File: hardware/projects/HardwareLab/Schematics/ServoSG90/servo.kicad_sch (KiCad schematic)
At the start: 2 parts

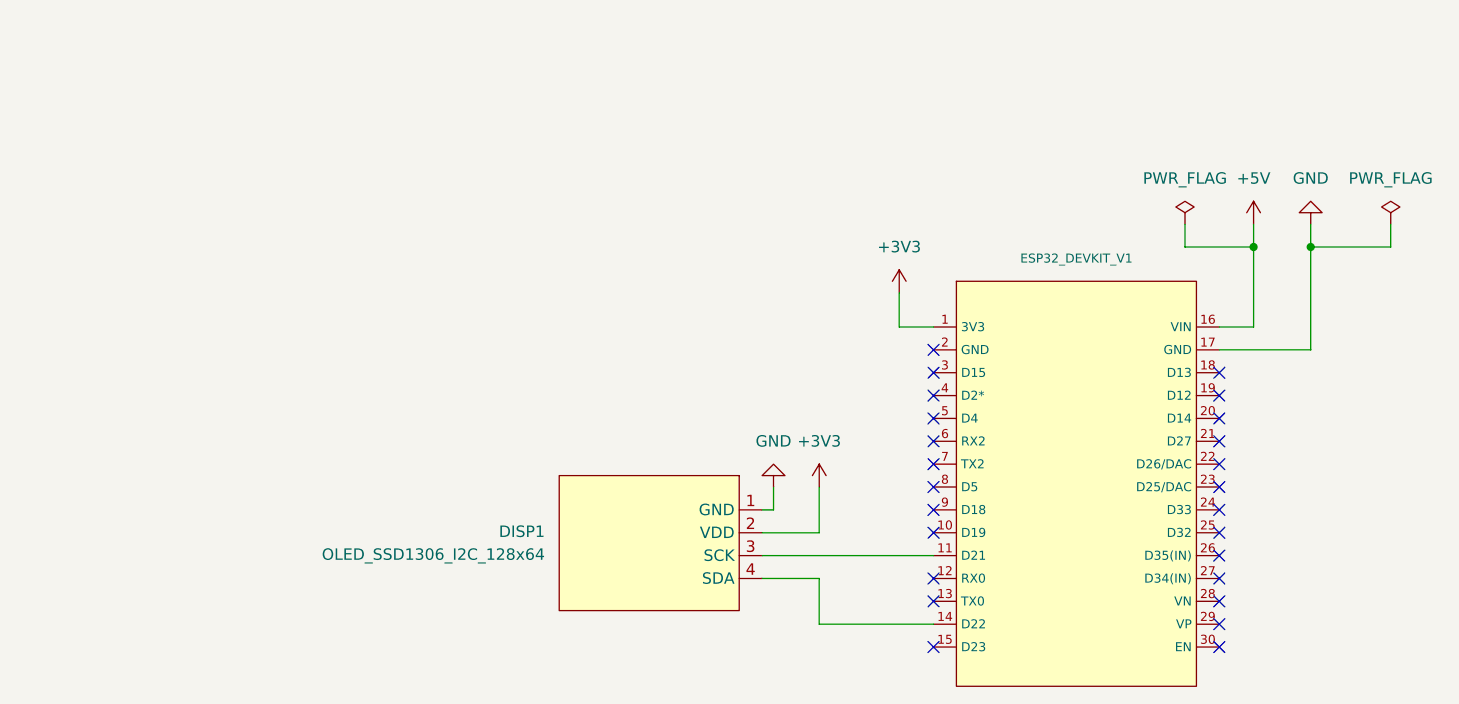
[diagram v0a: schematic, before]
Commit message: Inclusão do projeto de teste de Servo SG90
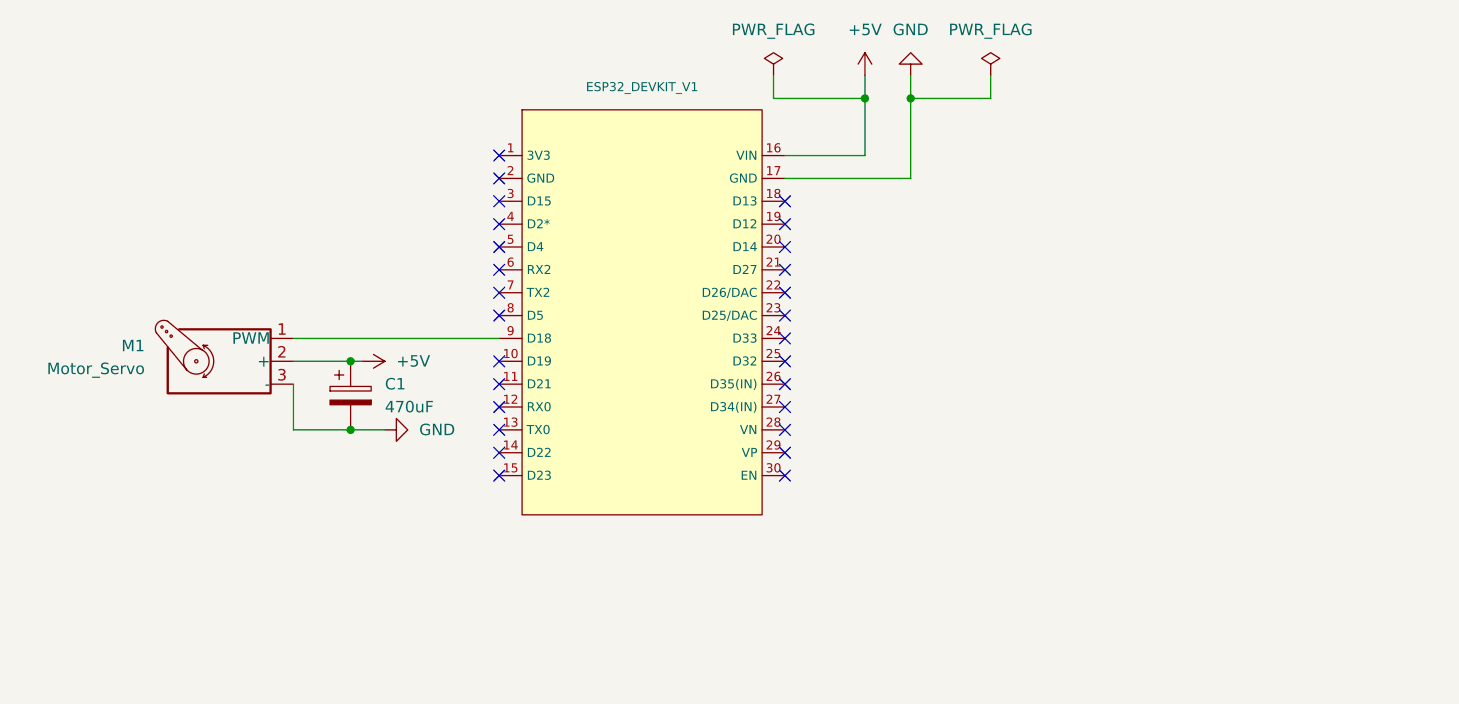
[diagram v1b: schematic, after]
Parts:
- removed DISP1: OLED_SSD1306_I2C_128x64, TechBaseLab:OLED_0.96_I2C_SSD1306_128x64, symbol TechBaseLab:OLED_SSD1306_I2C_128x64
- added C1: 470uF, symbol Device:C_Polarized
- added M1: Motor_Servo, symbol Motor:Motor_Servo
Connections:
- net +5V: now also C1.1, M1.2 (+)
- net GND: now also C1.2, M1.3 (-)
- net at ESP32_DEVKIT_V1.9 (D18): now also M1.1 (PWM)
- net +3V3: no longer names the net of ESP32_DEVKIT_V1.1 (3V3)
- no-connect marks 25 -> 27
